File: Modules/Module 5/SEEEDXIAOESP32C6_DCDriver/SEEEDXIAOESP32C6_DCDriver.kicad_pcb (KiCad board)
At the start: 2 copper layers, 47 x 22.8 mm, 8 parts, among them J1 Conn_01x07_Socket, J2 Conn_01x07_Socket, J3 Conn_01x02_Pin, J5 Conn_01x04_Pin, U1 TB6612FNG

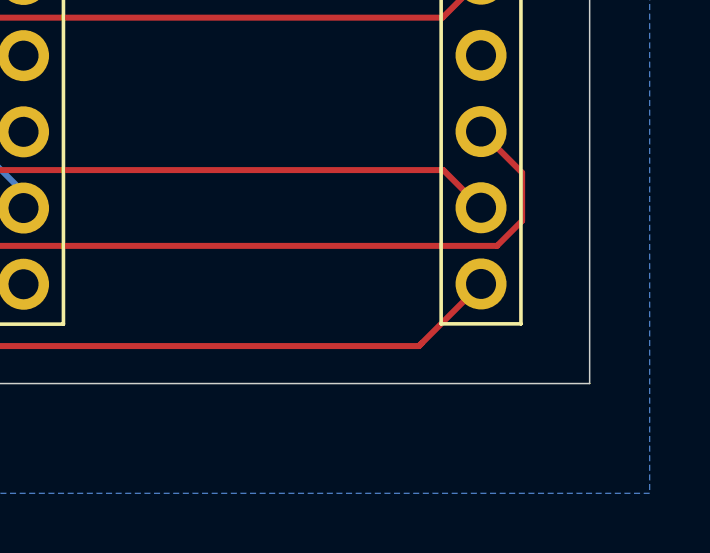
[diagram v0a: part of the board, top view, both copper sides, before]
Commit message: edits
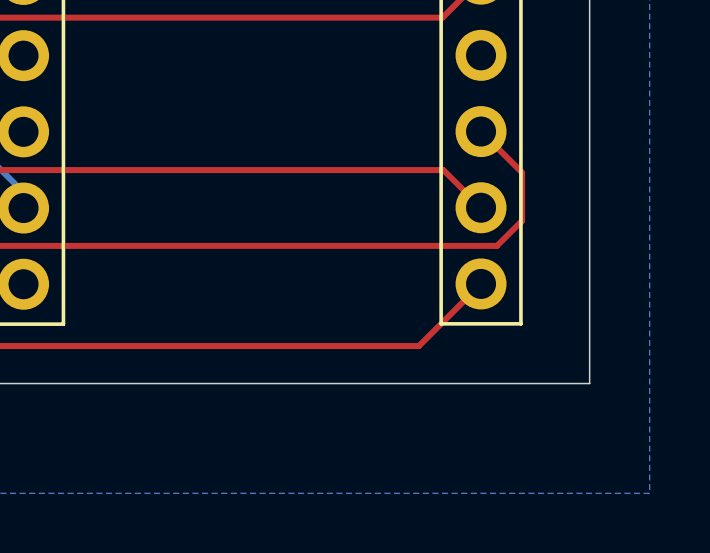
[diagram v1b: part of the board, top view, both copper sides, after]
